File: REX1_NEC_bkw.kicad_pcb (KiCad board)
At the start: 2 copper layers, 16 x 38 mm, 10 parts, among them J1 Molex_DIP28_edge_contacts, J2 JTAG, J3 PRG, U1 XCR3064XL-10VQ44, U2 29F800, U3 LP2980

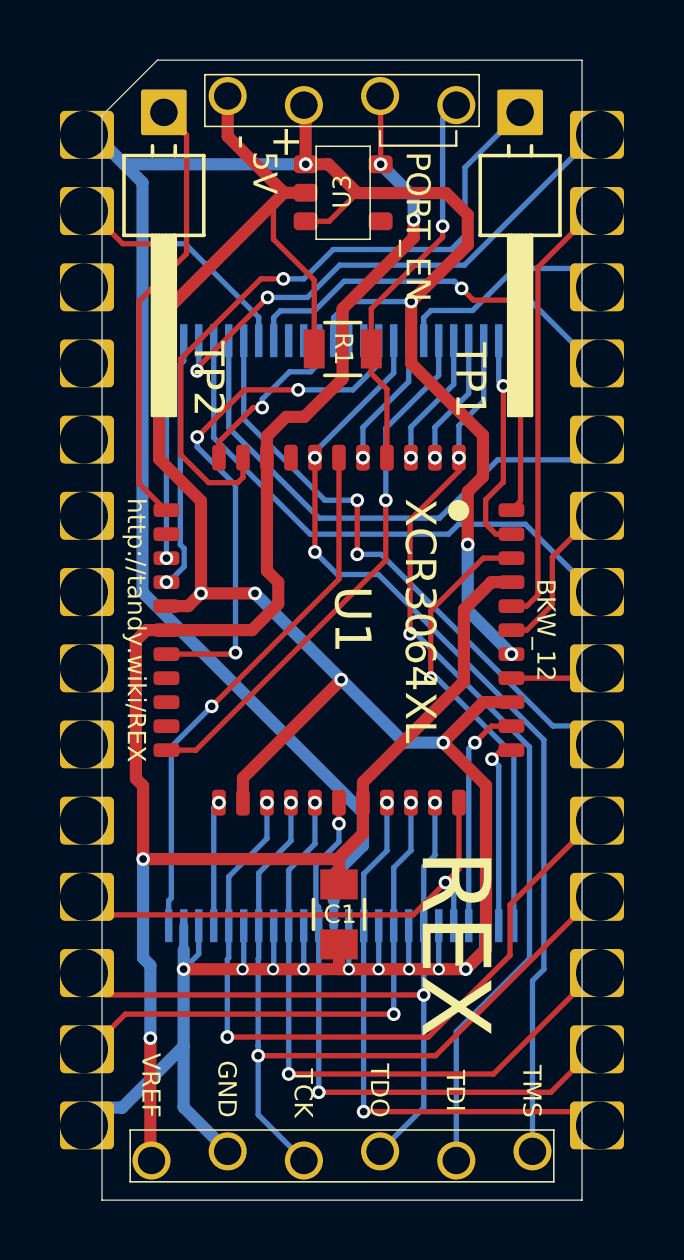
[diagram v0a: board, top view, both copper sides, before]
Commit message: initial NEC 8201a version
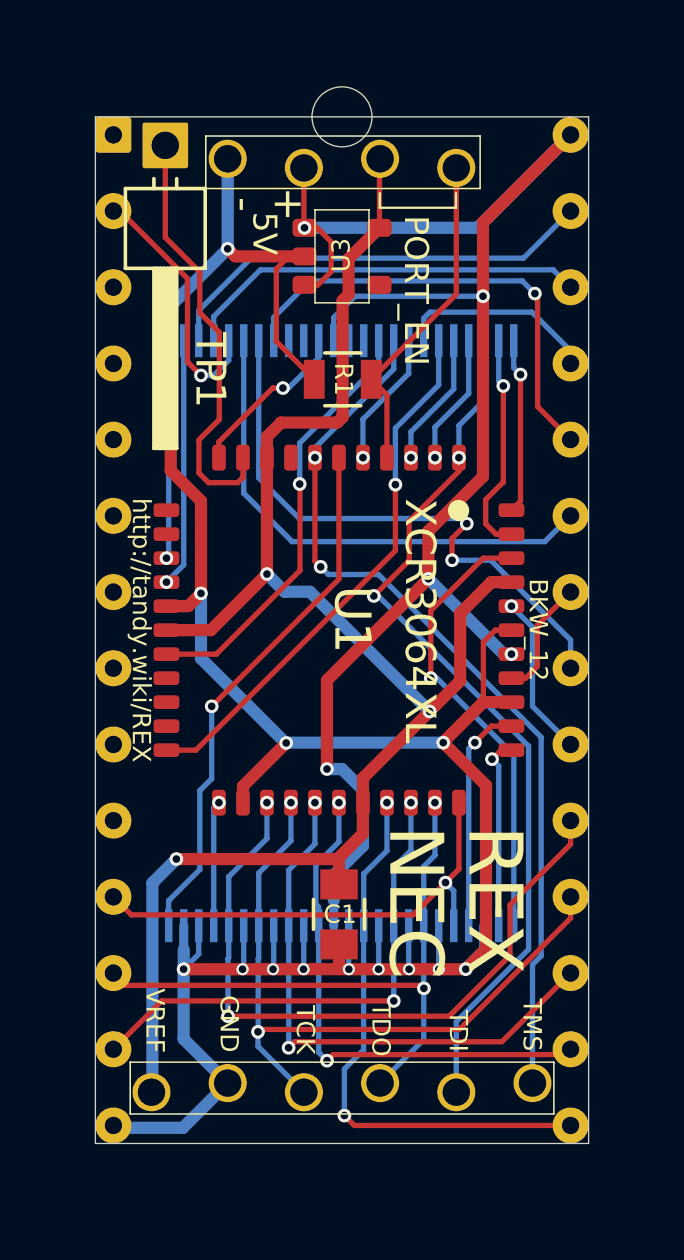
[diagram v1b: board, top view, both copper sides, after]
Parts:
- removed TP2: PINHD-1X1, 000_LOCAL:1x1_pin_h
- J1: value Molex_DIP28_edge_contacts -> DIP28_NEC_MAIN_ROM; footprint 000_LOCAL:pcb2molex8878_chamfer -> 000_LOCAL:DIP-28_W15.24mm_pcb_sil_pins
- moved TP1 11.9 mm to (141.3, 83.0)
- moved J2 2.28 mm to (147.2, 114.4)
- moved U3 2.12 mm to (147.2, 86.7)
- moved J3 2.09 mm to (147.2, 83.6)
- moved R1 1.01 mm to (147.2, 90.8)
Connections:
- J1 pad 1: /+5 -> (no net)
- J1 pad 2: /A10 -> /A12
- J1 pad 20: /A11 -> /~CS
- J1 pad 21: /~RD -> /A10
- J1 pad 22: /A13 -> /~RD
- J1 pad 23: /ALE -> /A11
- J1 pad 24: /A12 -> /A9
- J1 pad 25: /A9 -> /A8
- J1 pad 26: /A8 -> /A13
- J1 pad 27: /~CS -> /A14
- J1 pad 28: /A14 -> /+5
- U1 pad 12: /TP2 -> (no net)
- U1 pad 39: /ALE -> GND
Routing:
- net /TP2: track 14.6 -> 0.00 mm
- net /A10: track 8.07 -> 19.6 mm, vias 1 -> 2
- net /+5: track 69.6 -> 58.7 mm, vias 4 -> 5
- net /~CS: track 14.8 -> 5.43 mm, vias 0 -> 1
- net /A12: track 17.3 -> 8.61 mm, vias 0 -> 1
- net /TP1: track 22.4 -> 14.3 mm, vias 1 -> 0
- net +3V3: track 62.1 -> 54.4 mm, vias 4 -> 3
- net /ALE: track 5.48 -> 0.00 mm
- net /A13: track 18.5 -> 13.6 mm
- net /RY_BY: track 17.5 -> 14.0 mm, vias 3 -> 1
- net /AD1: track 24.0 -> 20.7 mm
- net /AD6: track 26.6 -> 23.4 mm
- net /A14: track 17.8 -> 14.8 mm, vias 2 -> 0
- net GND: track 90.3 -> 87.5 mm, vias 13 -> 14
- net /A11: track 19.7 -> 17.0 mm, vias 2 -> 0
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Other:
- board size 16 x 38 mm -> 16.4 x 34.2 mm
- board text added: "LEGS: TE 144242-1"
- board text added: "NEC"
